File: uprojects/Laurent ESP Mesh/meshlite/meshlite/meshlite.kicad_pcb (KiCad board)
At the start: 2 copper layers, 55.3 x 53.8 mm, 13 parts, among them J1 Conn_01x02, J2 Conn_01x02, J3 Conn_01x06, K1 CPC1916Y, U1 MOUDLE-SEEEDUINO-XIAO-ESP32C3

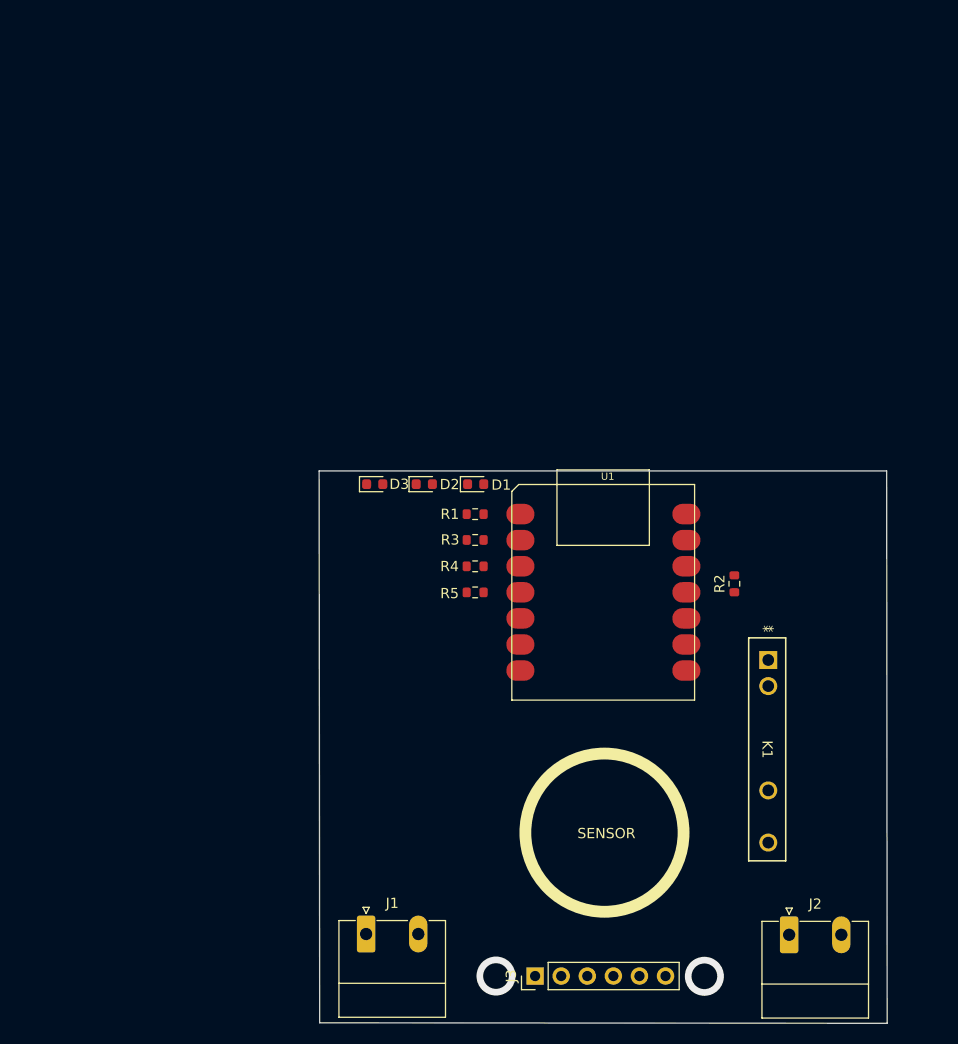
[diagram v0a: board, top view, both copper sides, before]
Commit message: 8-august 24
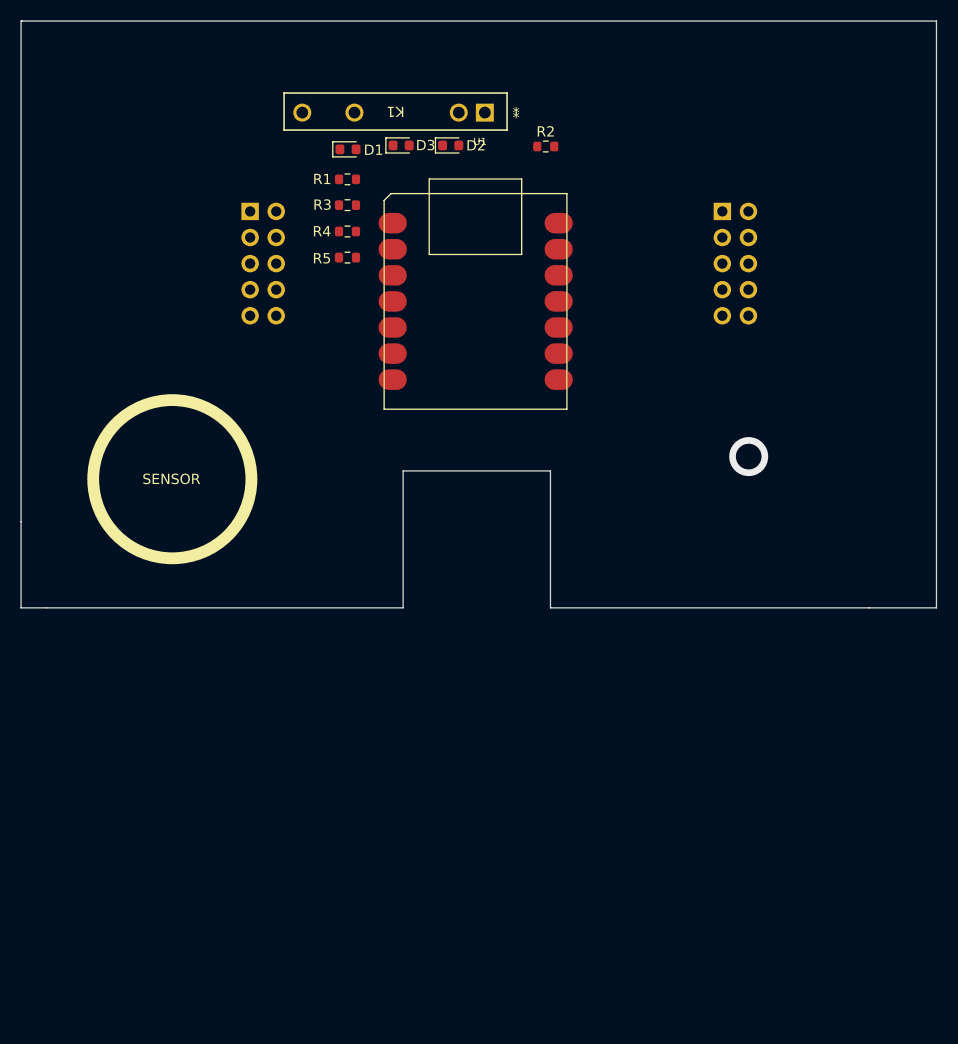
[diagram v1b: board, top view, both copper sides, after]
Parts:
- removed J1, J2: Conn_01x02, Connector_Phoenix_MC_HighVoltage:PhoenixContact_MC_1,5_2-G-5.08_1x02_P5.08mm_Horizontal
- added J4: Conn_02x05_Odd_Even, Connector_PinSocket_2.54mm:PinSocket_2x05_P2.54mm_Vertical, B.Cu at (114.9, 56.6)
- J3: value Conn_01x06 -> Conn_02x05_Odd_Even; footprint Connector_PinHeader_2.54mm:PinHeader_1x06_P2.54mm_Vertical -> Connector_PinSocket_2.54mm:PinSocket_2x05_P2.54mm_Vertical; moved to B.Cu
- moved J3 76.7 mm to (160.9, 56.6), turned to 180 degrees
- moved K1 60.0 mm to (137.8, 47.0), turned to 180 degrees
- moved R2 46.4 mm to (143.7, 50.3), turned to 0 degrees
- moved D1 34.9 mm to (124.4, 50.6)
- moved R4 34.9 mm to (124.4, 58.6)
- moved R5 34.9 mm to (124.4, 61.1)
- moved R1 34.9 mm to (124.4, 53.5)
- moved R3 34.9 mm to (124.4, 56.0)
- moved D2 33.1 mm to (134.4, 50.2)
- moved D3 33.1 mm to (129.6, 50.2)
- moved U1 30.9 mm to (127.9, 75.9)
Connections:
- K1 pad 3: Net-(J2-Pin_2) -> unconnected-(K1-Pad3)
- K1 pad 4: Net-(J2-Pin_1) -> unconnected-(K1-Pad4)
- R1 pad 1: Net-(J1-Pin_1) -> unconnected-(R1-Pad1)
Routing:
- net (no net): vias 2 -> 1
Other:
- board size 55.3 x 53.8 mm -> 89.2 x 57.1 mm
